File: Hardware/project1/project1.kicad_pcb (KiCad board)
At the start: 2 copper layers, 17 x 21.5 mm, 6 parts, among them J1 Conn_01x02, SW1 SW_Push_45deg

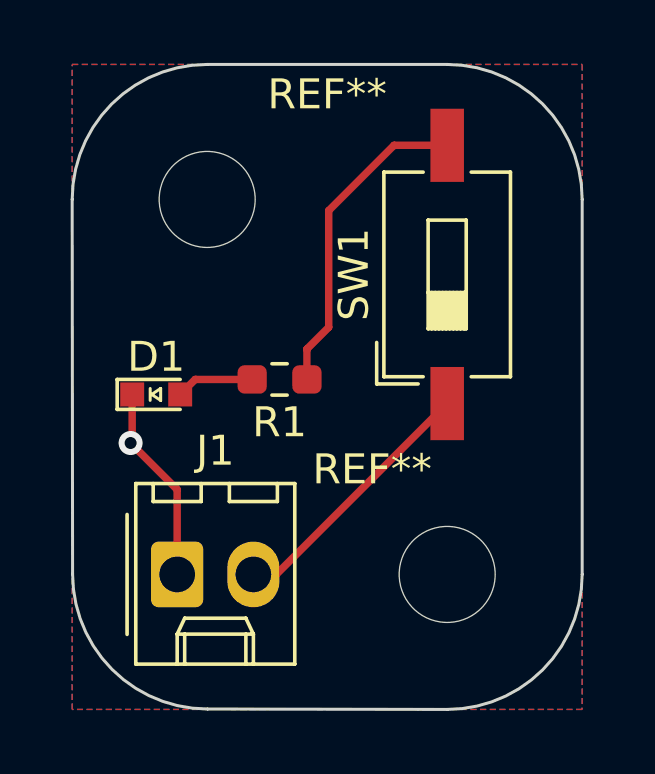
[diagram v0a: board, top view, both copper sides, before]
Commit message: Fixing hardware project 1 problems
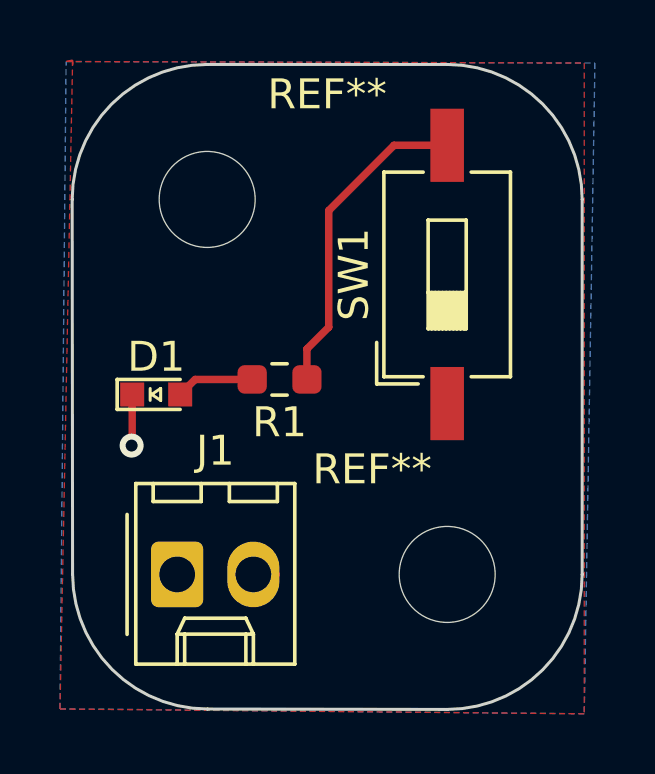
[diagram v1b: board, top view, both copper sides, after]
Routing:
- net +3V3: track 8.82 -> 0.76 mm
- net GND: track 6.66 -> 1.71 mm
- added copper zone on F.Cu, net +3V3
- removed copper zone on F.Cu, net (none)
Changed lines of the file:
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@@
 	)
 	(segment
-		(start 160.8003 114.9751)
-		(end 160.7479 115.0275)
+		(start 160.8003 113.4081)
+		(end 160.8003 115.0945)
 		(width 0.25)
 		(layer "F.Cu")
@@
 	)
 	(segment
-		(start 160.8003 113.4081)
-		(end 160.8003 114.9751)
-		(width 0.25)
-		(layer "F.Cu")
-		(net 1)
-	)
-	(segment
-		(start 162.3003 116.5799)
-		(end 160.7479 115.0275)
-		(width 0.25)
-		(layer "F.Cu")
-		(net 1)
-	)
-	(segment
-		(start 162.3003 119.4081)
-		(end 162.3003 116.5799)
+		(start 160.8003 115.0945)
+		(end 160.782 115.1128)
 		(width 0.25)
 		(layer "F.Cu")
@@
 	)
 	(via
-		(at 160.7479 115.0275)
+		(at 160.782 115.1128)
 		(size 0.8)
 		(drill 0.4)
@@
 		(net 4)
 	)
-	(segment
-		(start 165.6053 119.4081)
-		(end 171.3003 113.7131)
-		(width 0.25)
-		(layer "F.Cu")
+	(zone
 		(net 4)
-	)
-	(zone
-		(net 0)
-		(net_name "")
+		(net_name "+3V3")
 		(layer "F.Cu")
 		(hatch edge 0.5)
+		(priority 5)
 		(connect_pads
 			(clearance 0.508)
@@
 			(thermal_gap 0.5)
 			(thermal_bridge_width 0.5)
-			(island_removal_mode 1)
-			(island_area_min 10)
 		)
 		(polygon
 			(pts
-				(xy 158.8003 102.4081) (xy 175.8003 102.4081) (xy 175.8003 123.9081) (xy 158.8003 123.9081)
+				(xy 158.5976 102.3112) (xy 175.8696 102.362) (xy 175.8696 124.0536) (xy 158.3944 123.894395) (xy 158.814004 102.3112)
+				(xy 158.814004 102.4128) (xy 158.814004 102.2604)
 			)
 		)
@@
 		(polygon
 			(pts
-				(xy 158.8003 102.4081) (xy 175.8003 102.4081) (xy 175.8003 123.9081) (xy 158.8003 123.9081)
+				(xy 158.5976 102.3112) (xy 176.2252 102.362) (xy 175.8696 124.0536) (xy 158.3944 123.885953)
 			)
 		)
